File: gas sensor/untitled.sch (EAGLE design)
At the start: 34 parts, among them J1 POWER_JACKPTH

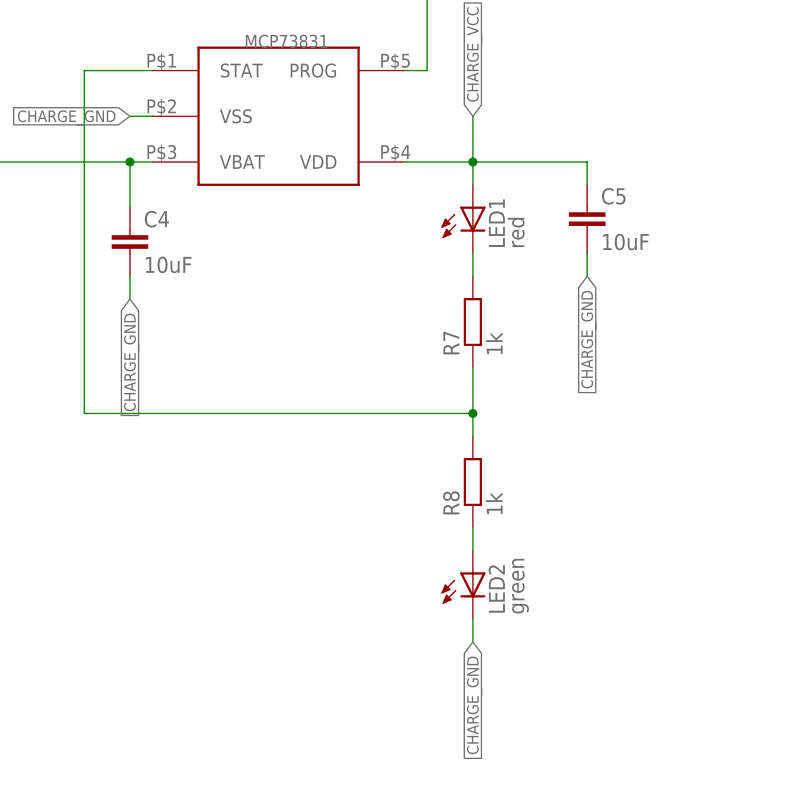
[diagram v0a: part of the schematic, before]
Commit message: gas sensor
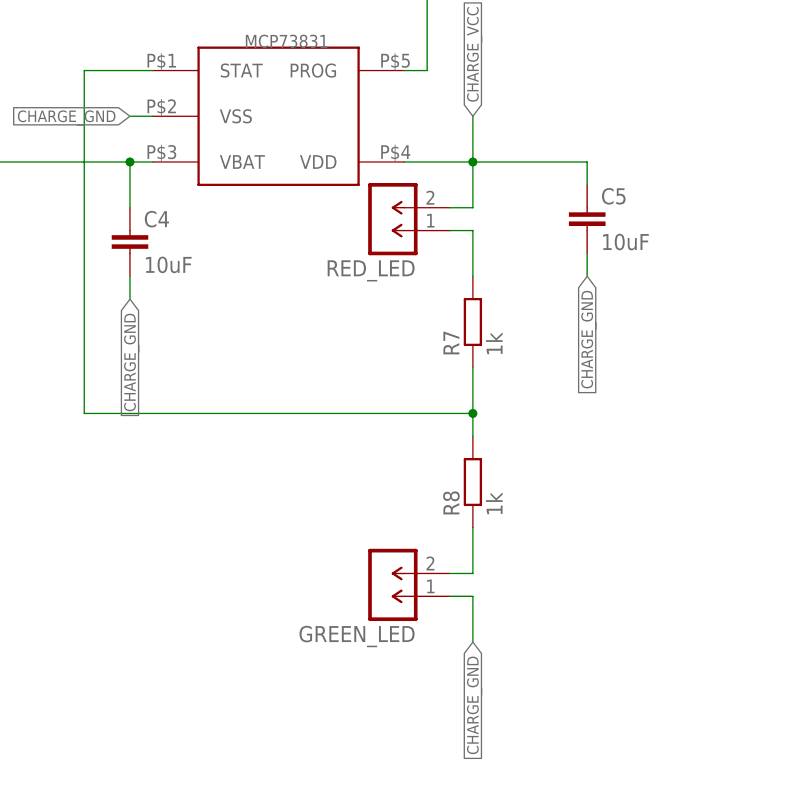
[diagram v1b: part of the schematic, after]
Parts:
- removed LED1: red, led:LEDCHIPLED_0805
- removed LED2: green, led:LEDCHIPLED_0805
- added GREEN_LED, RED_LED: M-1X02-SIP-100-32Y, con-headers-jp:M-1X02-SIP-100-32Y
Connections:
- net CHARGE_GND: now also GREEN_LED.1; no longer LED2.C
- net CHARGE_VCC: now also RED_LED.2; no longer LED1.A
- net N$1: now also GREEN_LED.2; no longer LED2.A
- net N$15: now also RED_LED.1; no longer LED1.C
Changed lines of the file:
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@@
 <?xml version="1.0" encoding="utf-8"?>
 <!DOCTYPE eagle SYSTEM "eagle.dtd">
-<eagle version="7.5.0">
+<eagle version="7.6.0">
 <drawing>
 <settings>
@@
 <part name="R7" library="resistor" deviceset="R-EU_" device="R1206" value="1k"/>
 <part name="R8" library="resistor" deviceset="R-EU_" device="R1206" value="1k"/>
-<part name="LED1" library="led" deviceset="LED" device="CHIPLED_0805" value="red"/>
-<part name="LED2" library="led" deviceset="LED" device="CHIPLED_0805" value="green"/>
 <part name="C4" library="resistor" deviceset="C-EU" device="C0805" value="10uF"/>
 <part name="C5" library="resistor" deviceset="C-EU" device="C0805" value="10uF"/>
@@
 <part name="SWITCH" library="con-headers-jp" deviceset="M-1X02-" device="SIP-100-32Y" value=""/>
 <part name="PIEZO" library="con-headers-jp" deviceset="M-1X02-" device="SIP-100-32Y" value=""/>
+<part name="RED_LED" library="con-headers-jp" deviceset="M-1X02-" device="SIP-100-32Y" value=""/>
+<part name="GREEN_LED" library="con-headers-jp" deviceset="M-1X02-" device="SIP-100-32Y" value=""/>
 </parts>
 <sheets>
@@
 <instance part="R7" gate="G$1" x="-96.52" y="-86.36" rot="R90"/>
 <instance part="R8" gate="G$1" x="-96.52" y="-104.14" rot="R90"/>
-<instance part="LED1" gate="G$1" x="-96.52" y="-73.66"/>
-<instance part="LED2" gate="G$1" x="-96.52" y="-114.3"/>
 <instance part="C4" gate="G$1" x="-134.62" y="-76.2"/>
 <instance part="C5" gate="G$1" x="-83.82" y="-73.66"/>
@@
 <instance part="SWITCH" gate="G$1" x="76.2" y="15.24" rot="R180"/>
 <instance part="PIEZO" gate="G$1" x="-35.56" y="40.64"/>
+<instance part="RED_LED" gate="G$1" x="-104.14" y="-76.2" rot="R180"/>
+<instance part="GREEN_LED" gate="G$1" x="-104.14" y="-116.84" rot="R180"/>
 </instances>
 <busses>
@@
 <pinref part="MCP73831" gate="G$1" pin="VDD"/>
 <wire x1="-83.82" y1="-68.58" x2="-96.52" y2="-68.58" width="0.1524" layer="91"/>
-<pinref part="LED1" gate="G$1" pin="A"/>
 <wire x1="-96.52" y1="-68.58" x2="-104.14" y2="-68.58" width="0.1524" layer="91"/>
-<wire x1="-96.52" y1="-71.12" x2="-96.52" y2="-68.58" width="0.1524" layer="91"/>
 <junction x="-96.52" y="-68.58"/>
 <wire x1="-96.52" y1="-68.58" x2="-96.52" y2="-63.5" width="0.1524" layer="91"/>
 <label x="-96.52" y="-63.5" size="1.27" layer="95" rot="R90" xref="yes"/>
+<pinref part="RED_LED" gate="G$1" pin="2"/>
+<wire x1="-99.06" y1="-73.66" x2="-96.52" y2="-73.66" width="0.1524" layer="91"/>
+<wire x1="-96.52" y1="-73.66" x2="-96.52" y2="-68.58" width="0.1524" layer="91"/>
 </segment>
 </net>
@@
 </segment>
 <segment>
-<wire x1="-96.52" y1="-119.38" x2="-96.52" y2="-121.92" width="0.1524" layer="91"/>
 <label x="-96.52" y="-121.92" size="1.27" layer="95" rot="R270" xref="yes"/>
-<pinref part="LED2" gate="G$1" pin="C"/>
+<pinref part="GREEN_LED" gate="G$1" pin="1"/>
+<wire x1="-99.06" y1="-116.84" x2="-96.52" y2="-116.84" width="0.1524" layer="91"/>
+<wire x1="-96.52" y1="-116.84" x2="-96.52" y2="-121.92" width="0.1524" layer="91"/>
 </segment>
 <segment>
@@
 <net name="N$15" class="0">
 <segment>
-<pinref part="LED1" gate="G$1" pin="C"/>
 <pinref part="R7" gate="G$1" pin="2"/>
-<wire x1="-96.52" y1="-78.74" x2="-96.52" y2="-81.28" width="0.1524" layer="91"/>
+<pinref part="RED_LED" gate="G$1" pin="1"/>
+<wire x1="-99.06" y1="-76.2" x2="-96.52" y2="-76.2" width="0.1524" layer="91"/>
+<wire x1="-96.52" y1="-76.2" x2="-96.52" y2="-81.28" width="0.1524" layer="91"/>
 </segment>
 </net>
@@
 <net name="N$1" class="0">
 <segment>
-<pinref part="LED2" gate="G$1" pin="A"/>
 <pinref part="R8" gate="G$1" pin="1"/>
-<wire x1="-96.52" y1="-111.76" x2="-96.52" y2="-109.22" width="0.1524" layer="91"/>
-</segment>
-</net>
+<wire x1="-96.52" y1="-109.22" x2="-96.52" y2="-114.3" width="0.1524" layer="91"/>
+<pinref part="GREEN_LED" gate="G$1" pin="2"/>
+<wire x1="-96.52" y1="-114.3" x2="-99.06" y2="-114.3" width="0.1524" layer="91"/>
+</segment>
+</net>
